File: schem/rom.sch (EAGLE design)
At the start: 14 parts, among them IC10 74HC32N, IC11 74HC32N, IC12 74HC32N, IC13 74HC32N, IC14 74HC04N, IC6 74HC374N, IC7 74HC08N, IC8 74HC377N, IC9 74HC377N

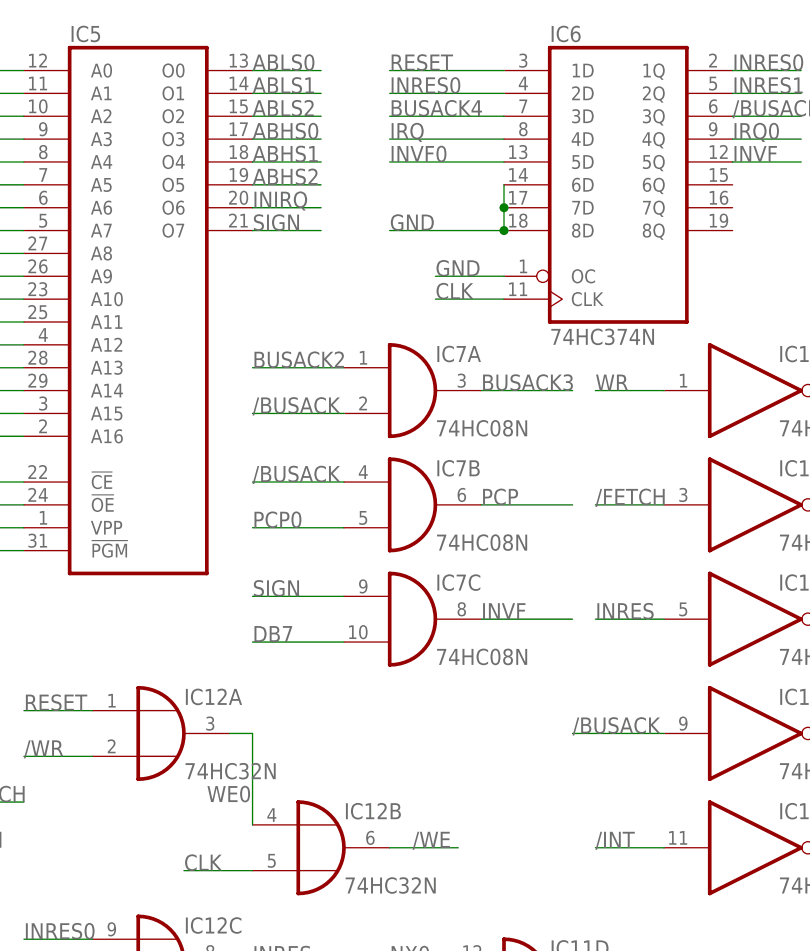
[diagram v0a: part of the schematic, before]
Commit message: progress
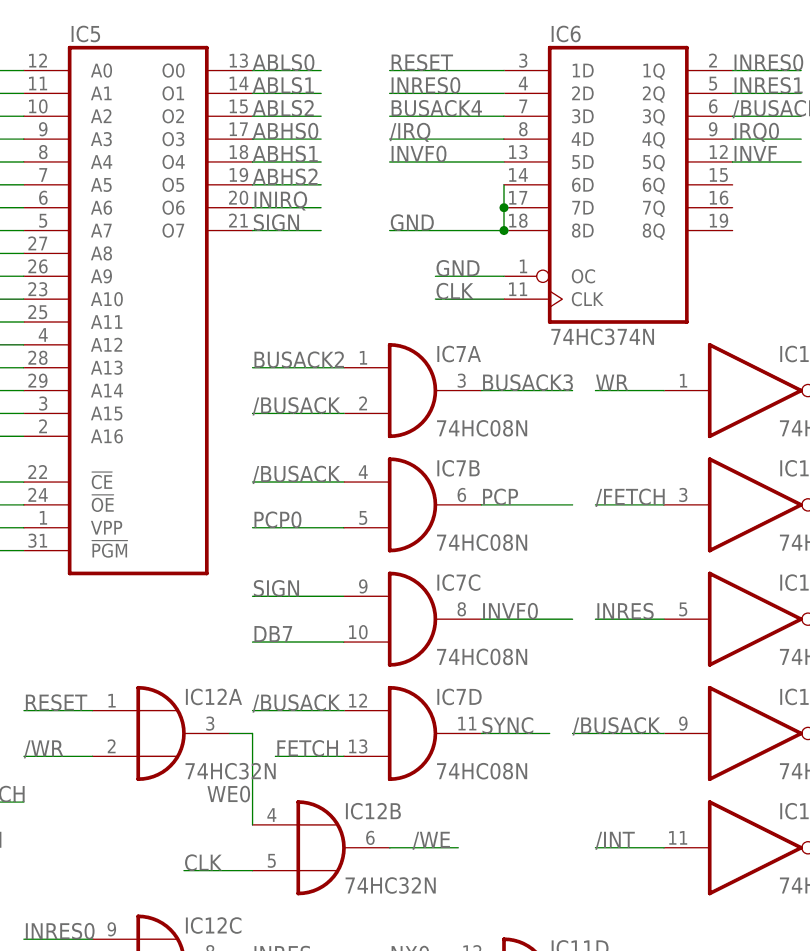
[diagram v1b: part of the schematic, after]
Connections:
- net IRQ renamed /IRQ
- new net SYNC: IC7D.O
- net /BUSACK: now also IC7D.I0
- net FETCH: now also IC7D.I1
- net INVF: no longer IC7C.O
- net INVF0: now also IC7C.O
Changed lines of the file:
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@@
 <instance part="IC13" gate="B" x="269.24" y="-15.24"/>
 <instance part="IC13" gate="C" x="154.94" y="-20.32"/>
+<instance part="IC7" gate="D" x="228.6" y="20.32"/>
 </instances>
 <busses>
@@
 </segment>
 </net>
-<net name="IRQ" class="0">
+<net name="/IRQ" class="0">
 <segment>
 <pinref part="IC6" gate="A" pin="4D"/>
@@
 <wire x1="220.98" y1="48.26" x2="210.82" y2="48.26" width="0.1524" layer="91"/>
 <label x="210.82" y="48.26" size="1.778" layer="95"/>
+</segment>
+<segment>
+<pinref part="IC7" gate="D" pin="I0"/>
+<wire x1="220.98" y1="22.86" x2="210.82" y2="22.86" width="0.1524" layer="91"/>
+<label x="210.82" y="22.86" size="1.778" layer="95"/>
 </segment>
 </net>
@@
 <label x="276.86" y="45.72" size="1.778" layer="95"/>
 </segment>
+<segment>
+<pinref part="IC7" gate="D" pin="I1"/>
+<wire x1="220.98" y1="17.78" x2="213.36" y2="17.78" width="0.1524" layer="91"/>
+<label x="213.36" y="17.78" size="1.778" layer="95"/>
+</segment>
 </net>
 <net name="/INRES" class="0">
@@
 <label x="226.06" y="83.82" size="1.778" layer="95"/>
 </segment>
+<segment>
+<pinref part="IC7" gate="C" pin="O"/>
+<wire x1="236.22" y1="33.02" x2="246.38" y2="33.02" width="0.1524" layer="91"/>
+<label x="236.22" y="33.02" size="1.778" layer="95"/>
+</segment>
 </net>
 <net name="INVF" class="0">
@@
 <label x="264.16" y="83.82" size="1.778" layer="95"/>
 </segment>
-<segment>
-<pinref part="IC7" gate="C" pin="O"/>
-<wire x1="236.22" y1="33.02" x2="246.38" y2="33.02" width="0.1524" layer="91"/>
-<label x="236.22" y="33.02" size="1.778" layer="95"/>
-</segment>
-</net>
+</net>
+<net name="SYNC" class="0">
+<segment>
+<pinref part="IC7" gate="D" pin="O"/>
+<wire x1="236.22" y1="20.32" x2="243.84" y2="20.32" width="0.1524" layer="91"/>
+<label x="236.22" y="20.32" size="1.778" layer="95"/>
+</segment>
+</net>

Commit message: board changes ; rom schematic finished
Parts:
- added SV1, SV3, SV4, SV6, SV7, SV8: (no value), con-lstb:MA08-1
- added SV10, SV2, SV5, SV9: (no value), con-lstb:MA06-1
- added SV11, SV12, SV13: (no value), con-lstb:MA05-2
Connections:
- removed net IBS0: IC2A.O0
- removed net IBS1: IC2A.O1
- removed net IBS2: IC2A.O2
- removed net IBS3: IC2A.O3
- new net IB0: SV1.1
- new net IB1: SV1.2
- new net IB2: SV1.3
- new net IB3: SV1.4
- new net IB4: SV1.5
- new net IB5: SV1.6
- new net IB6: SV1.7
- new net IB7: SV1.8
- new net IBR0: IC2A.O0, SV10.3
- new net IBR1: IC2A.O1, SV10.4
- new net IBR2: IC2A.O2, SV10.5
- new net IBR3: IC2A.O3, SV10.6
- new net OB0: SV4.1
- new net OB1: SV4.2
- new net OB2: SV4.3
- new net OB3: SV4.4
- new net OB4: SV4.5
- new net OB5: SV4.6
- new net OB6: SV4.7
- new net OB7: SV4.8
- net /BUSACK: now also SV9.2
- net /BUSREQ: now also SV9.3
- net /INRES: now also SV12.3
- net /IRQ: now also SV9.6
- net /WE: now also SV9.4
- net ABHS0: now also SV11.2
- net ABHS1: now also SV11.4
- net ABHS2: now also SV11.6
- net ABLS0: now also SV12.2
- net ABLS1: now also SV12.4
- net ABLS2: now also SV12.6
- net ALUC: now also SV8.3
- net BUSACK: now also SV9.1
- net CIN: now also SV6.8
- net CLK: now also SV2.3
- net COND: now also SV8.7
- net DB0: now also SV3.1
- net DB1: now also SV3.2
- net DB2: now also SV3.3
- net DB3: now also SV3.4
- net DB4: now also SV3.5
- net DB5: now also SV3.6
- net DB6: now also SV3.7
- net DB7: now also SV3.8
- net DP: now also SV12.1
- net F0: now also SV6.1
- net F1: now also SV6.2
- net F2: now also SV6.3
- net F3: now also SV6.4
- net F4: now also SV6.5
- net F5: now also SV6.6
- net FL0: now also SV7.1
- net FL1: now also SV7.2
- net FL2: now also SV7.3
- net FL3: now also SV7.4
- net FL4: now also SV7.5
- net FL5: now also SV7.6
- net FL6: now also SV7.7
- net FL7: now also SV7.8
- net FL8: now also SV8.1
- net FL9: now also SV8.2
- net GND: now also IC13D.I0, IC13D.I1, IC14F.I, SV11.10, SV11.9, SV12.10, SV12.5, SV12.7, SV12.9, SV13.10, SV13.9, SV2.4, SV2.5, SV2.6, SV5.4, SV5.5, SV5.6, SV8.8
- net IN0: now also SV13.1
- net IN1: now also SV13.2
- net IN2: now also SV13.3
- net IN3: now also SV13.4
- net IN4: now also SV13.5
- net IN5: now also SV13.6
- net IN6: now also SV13.7
- net IN7: now also SV13.8
- net INIRQ: now also SV8.6
- net INVF: now also SV6.7
- net OBS0: now also SV11.1
- net OBS1: now also SV11.3
- net OBS2: now also SV11.5
- net OBS3: now also SV11.7
- net PCP: now also SV11.8, SV12.8
- net PQ0: now also SV8.4
- net PQ2: now also SV8.5
- net RESET: now also SV10.1
- net SYNC: now also SV10.2
- net VCC: now also SV2.1, SV2.2, SV5.1, SV5.2, SV5.3
- net WR: now also SV9.5
